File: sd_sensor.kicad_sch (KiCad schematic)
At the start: 12 parts, among them J401 SHOU HAN TF-CARD H1.8, U401 TMP102xxDRL

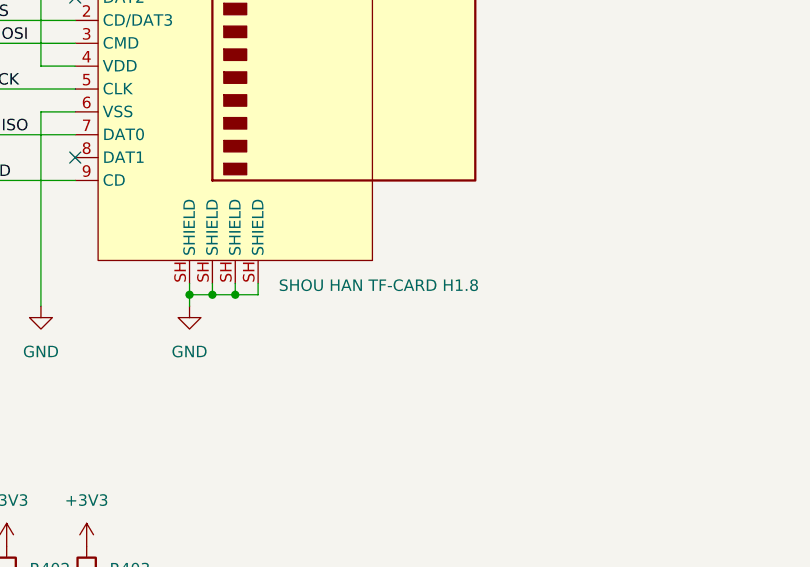
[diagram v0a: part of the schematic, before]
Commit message: Vérification des règles électriques
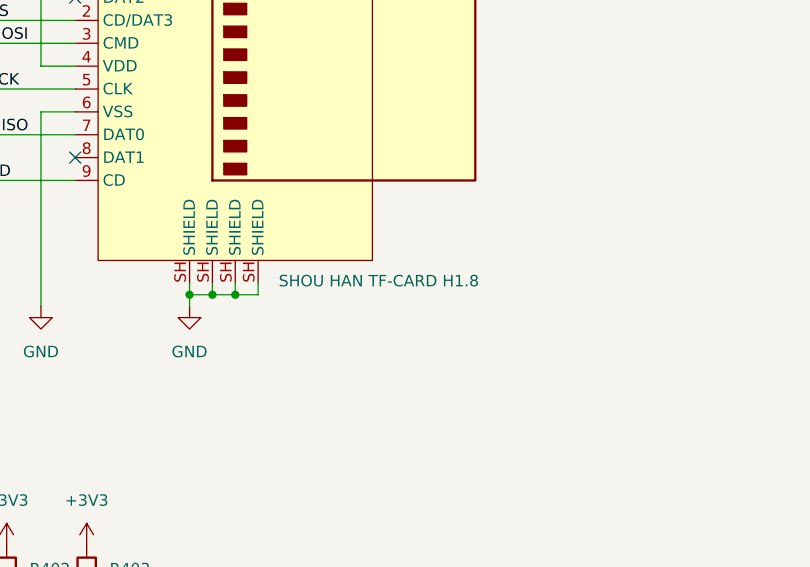
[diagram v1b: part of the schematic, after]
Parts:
- C401, C402: footprint (none) -> Capacitor_SMD:C_0402_1005Metric
- R401, R402, R403: footprint (none) -> Resistor_SMD:R_0402_1005Metric
- TP401, TP402, TP403, TP404, TP405: footprint (none) -> TestPoint:TestPoint_Pad_D2.0mm
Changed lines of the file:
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@@
 			)
 		)
-		(property "Footprint" ""
+		(property "Footprint" "TestPoint:TestPoint_Pad_D2.0mm"
 			(at 69.85 160.02 0)
 			(effects
@@
 			)
 		)
-		(property "Footprint" ""
+		(property "Footprint" "Capacitor_SMD:C_0402_1005Metric"
 			(at 49.2252 60.96 0)
 			(effects
@@
 			)
 		)
-		(property "Footprint" ""
+		(property "Footprint" "Resistor_SMD:R_0402_1005Metric"
 			(at 52.832 137.16 90)
 			(effects
@@
 			)
 		)
-		(property "Footprint" ""
+		(property "Footprint" "TestPoint:TestPoint_Pad_D2.0mm"
 			(at 69.85 157.48 0)
 			(effects
@@
 			)
 		)
-		(property "Footprint" ""
+		(property "Footprint" "TestPoint:TestPoint_Pad_D2.0mm"
 			(at 69.85 152.4 0)
 			(effects
@@
 			)
 		)
-		(property "Footprint" ""
+		(property "Footprint" "TestPoint:TestPoint_Pad_D2.0mm"
 			(at 69.85 154.94 0)
 			(effects
@@
 			)
 		)
-		(property "Footprint" ""
+		(property "Footprint" "Resistor_SMD:R_0402_1005Metric"
 			(at 202.692 59.69 90)
 			(effects
@@
 			)
 		)
-		(property "Footprint" ""
+		(property "Footprint" "TestPoint:TestPoint_Pad_D2.0mm"
 			(at 69.85 149.86 0)
 			(effects
@@
 			)
 		)
-		(property "Footprint" ""
+		(property "Footprint" "Capacitor_SMD:C_0402_1005Metric"
 			(at 205.4352 73.66 0)
 			(effects
@@
 			)
 		)
-		(property "Footprint" ""
+		(property "Footprint" "Resistor_SMD:R_0402_1005Metric"
 			(at 61.722 137.16 90)
 			(effects
@@
 		)
 		(property "Value" "SHOU HAN TF-CARD H1.8"
-			(at 84.836 104.394 0)
-			(effects
-				(font
+			(at 84.836 103.886 0)
+			(effects
+				(font
